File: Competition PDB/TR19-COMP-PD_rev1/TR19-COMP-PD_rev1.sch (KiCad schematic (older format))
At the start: 38 parts

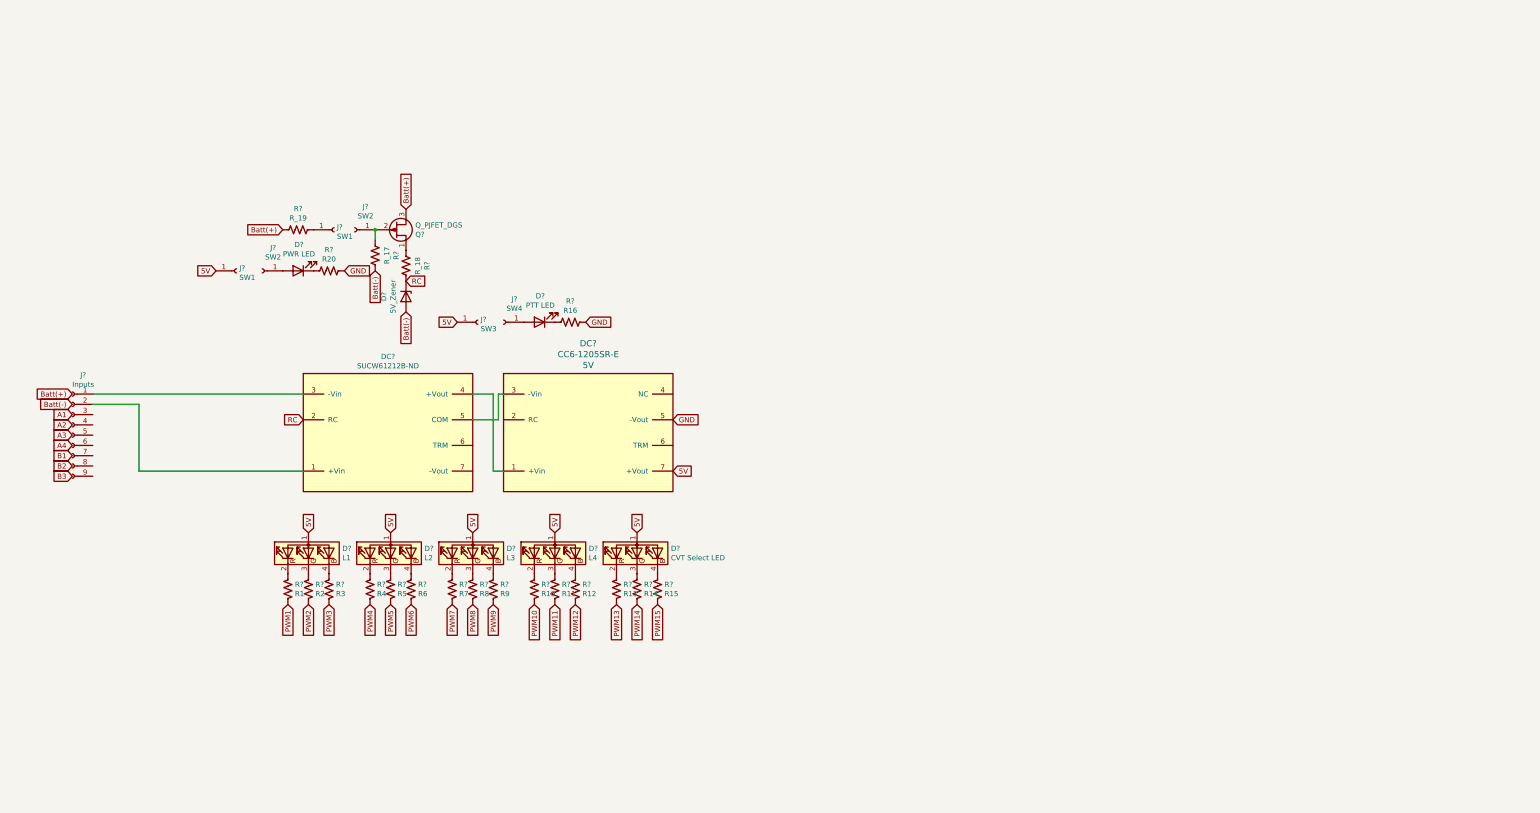
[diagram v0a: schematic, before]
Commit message: Baja Competition PCBs
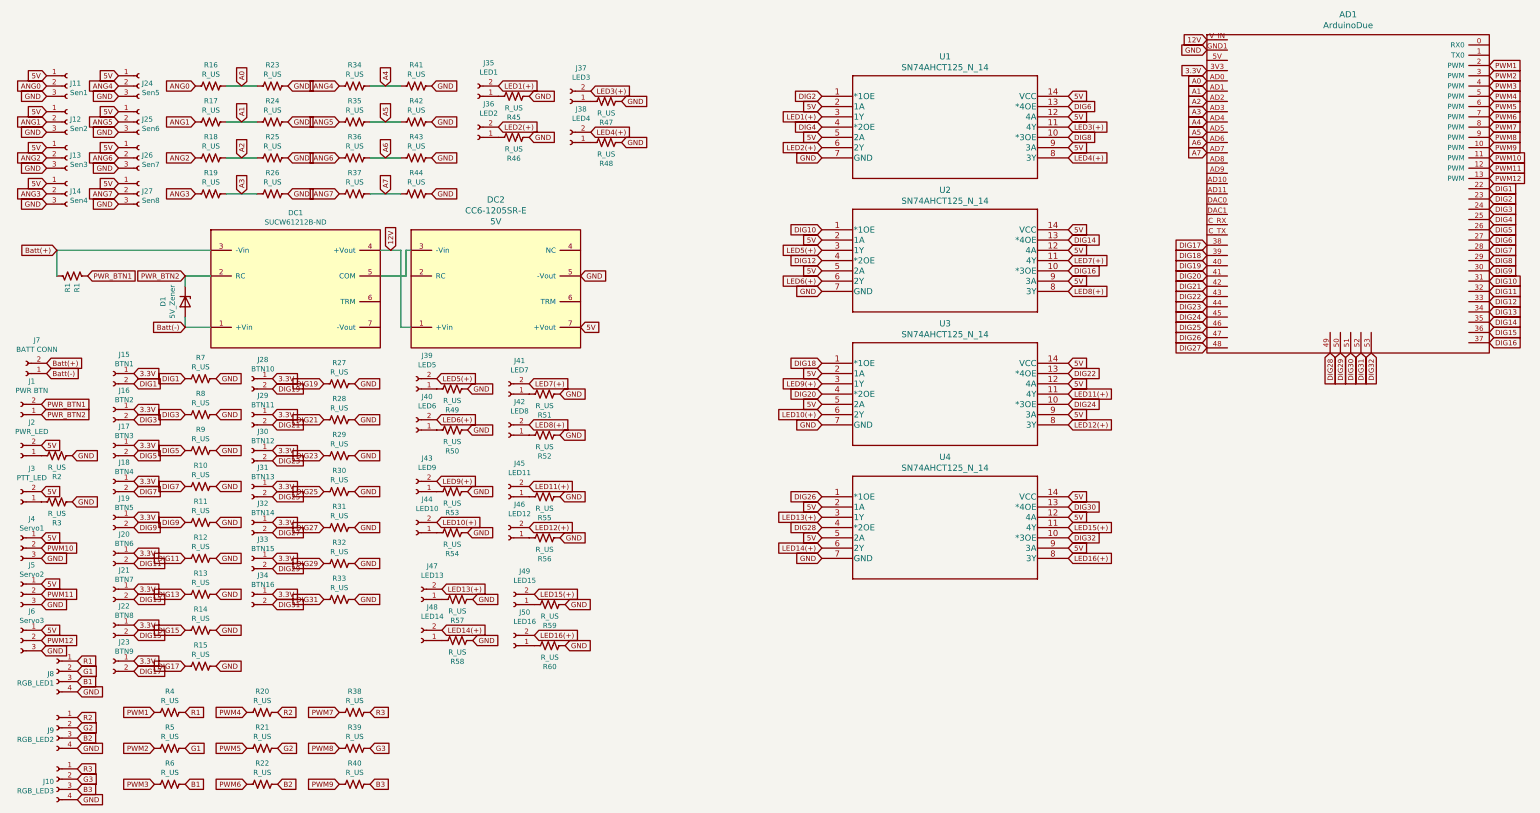
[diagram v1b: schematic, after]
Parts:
- removed D?: 5V_Zener, symbol Device:D_Zener
- removed D?: L1, symbol Device:LED_ARGB
- removed D?: L2, symbol Device:LED_ARGB
- removed D?: L3, symbol Device:LED_ARGB
- removed D?: L4, symbol Device:LED_ARGB
- removed D?: CVT Select LED, symbol Device:LED_ARGB
- removed D?: PTT LED, symbol Device:LED
- removed D?: PWR LED, symbol Device:LED
- removed J? (x2): SW1, symbol Connector:Conn_01x01_Female
- removed J? (x2): SW2, symbol Connector:Conn_01x01_Female
- removed J?: Inputs, symbol Connector:Conn_01x09_Female
- removed J?: SW3, symbol Connector:Conn_01x01_Female
- removed J?: SW4, symbol Connector:Conn_01x01_Female
- removed Q?: Q_PJFET_DGS, symbol Device:Q_PJFET_DGS
- removed R?: R_19, symbol Device:R_US
- removed R?: R1, symbol Device:R_US
- removed R?: R2, symbol Device:R_US
- removed R?: R3, symbol Device:R_US
- removed R?: R4, symbol Device:R_US
- removed R?: R5, symbol Device:R_US
- removed R?: R6, symbol Device:R_US
- removed R?: R7, symbol Device:R_US
- removed R?: R8, symbol Device:R_US
- removed R?: R9, symbol Device:R_US
- removed R?: R10, symbol Device:R_US
- removed R?: R11, symbol Device:R_US
- removed R?: R12, symbol Device:R_US
- removed R?: R13, symbol Device:R_US
- removed R?: R14, symbol Device:R_US
- removed R?: R15, symbol Device:R_US
- removed R?: R16, symbol Device:R_US
- removed R?: R_17, symbol Device:R_US
- removed R?: R_18, symbol Device:R_US
- removed R?: R20, symbol Device:R_US
- added AD1: ArduinoDue, TR_Library:ARDUINO_DUE_SHIELD_V2, symbol TR-Baja-Components:ArduinoDue
- added D1: 5V_Zener, Diode_SMD:D_0603_1608Metric_Pad1.05x0.95mm_HandSolder, symbol Device:D_Zener
- added J1: PWR BTN, Connector_PinHeader_2.54mm:PinHeader_1x02_P2.54mm_Vertical, symbol Connector:Conn_01x02_Female
- added J10: RGB_LED3, Connector_PinHeader_2.54mm:PinHeader_1x04_P2.54mm_Vertical, symbol Connector:Conn_01x04_Female
- added J11: Sen1, Connector_PinHeader_2.54mm:PinHeader_1x03_P2.54mm_Vertical, symbol Connector:Conn_01x03_Female
- added J12: Sen2, Connector_PinHeader_2.54mm:PinHeader_1x03_P2.54mm_Vertical, symbol Connector:Conn_01x03_Female
- added J13: Sen3, Connector_PinHeader_2.54mm:PinHeader_1x03_P2.54mm_Vertical, symbol Connector:Conn_01x03_Female
- added J14: Sen4, Connector_PinHeader_2.54mm:PinHeader_1x03_P2.54mm_Vertical, symbol Connector:Conn_01x03_Female
- added J15: BTN1, Connector_PinHeader_2.54mm:PinHeader_1x02_P2.54mm_Vertical, symbol Connector:Conn_01x02_Female
- added J16: BTN2, Connector_PinHeader_2.54mm:PinHeader_1x02_P2.54mm_Vertical, symbol Connector:Conn_01x02_Female
- added J17: BTN3, Connector_PinHeader_2.54mm:PinHeader_1x02_P2.54mm_Vertical, symbol Connector:Conn_01x02_Female
- added J18: BTN4, Connector_PinHeader_2.54mm:PinHeader_1x02_P2.54mm_Vertical, symbol Connector:Conn_01x02_Female
- added J19: BTN5, Connector_PinHeader_2.54mm:PinHeader_1x02_P2.54mm_Vertical, symbol Connector:Conn_01x02_Female
- added J2: PWR_LED, Connector_PinHeader_2.54mm:PinHeader_1x02_P2.54mm_Vertical, symbol Connector:Conn_01x02_Female
- added J20: BTN6, Connector_PinHeader_2.54mm:PinHeader_1x02_P2.54mm_Vertical, symbol Connector:Conn_01x02_Female
- added J21: BTN7, Connector_PinHeader_2.54mm:PinHeader_1x02_P2.54mm_Vertical, symbol Connector:Conn_01x02_Female
- added J22: BTN8, Connector_PinHeader_2.54mm:PinHeader_1x02_P2.54mm_Vertical, symbol Connector:Conn_01x02_Female
- added J23: BTN9, Connector_PinHeader_2.54mm:PinHeader_1x02_P2.54mm_Vertical, symbol Connector:Conn_01x02_Female
- added J24: Sen5, Connector_PinHeader_2.54mm:PinHeader_1x03_P2.54mm_Vertical, symbol Connector:Conn_01x03_Female
- added J25: Sen6, Connector_PinHeader_2.54mm:PinHeader_1x03_P2.54mm_Vertical, symbol Connector:Conn_01x03_Female
- added J26: Sen7, Connector_PinHeader_2.54mm:PinHeader_1x03_P2.54mm_Vertical, symbol Connector:Conn_01x03_Female
- added J27: Sen8, Connector_PinHeader_2.54mm:PinHeader_1x03_P2.54mm_Vertical, symbol Connector:Conn_01x03_Female
- added J28: BTN10, Connector_PinHeader_2.54mm:PinHeader_1x02_P2.54mm_Vertical, symbol Connector:Conn_01x02_Female
- added J29: BTN11, Connector_PinHeader_2.54mm:PinHeader_1x02_P2.54mm_Vertical, symbol Connector:Conn_01x02_Female
- added J3: PTT_LED, Connector_PinHeader_2.54mm:PinHeader_1x02_P2.54mm_Vertical, symbol Connector:Conn_01x02_Female
- added J30: BTN12, Connector_PinHeader_2.54mm:PinHeader_1x02_P2.54mm_Vertical, symbol Connector:Conn_01x02_Female
- added J31: BTN13, Connector_PinHeader_2.54mm:PinHeader_1x02_P2.54mm_Vertical, symbol Connector:Conn_01x02_Female
- added J32: BTN14, Connector_PinHeader_2.54mm:PinHeader_1x02_P2.54mm_Vertical, symbol Connector:Conn_01x02_Female
- added J33: BTN15, Connector_PinHeader_2.54mm:PinHeader_1x02_P2.54mm_Vertical, symbol Connector:Conn_01x02_Female
- added J34: BTN16, Connector_PinHeader_2.54mm:PinHeader_1x02_P2.54mm_Vertical, symbol Connector:Conn_01x02_Female
- added J35: LED1, Connector_PinHeader_2.54mm:PinHeader_1x02_P2.54mm_Vertical, symbol Connector:Conn_01x02_Female
- added J36: LED2, Connector_PinHeader_2.54mm:PinHeader_1x02_P2.54mm_Vertical, symbol Connector:Conn_01x02_Female
- added J37: LED3, Connector_PinHeader_2.54mm:PinHeader_1x02_P2.54mm_Vertical, symbol Connector:Conn_01x02_Female
- added J38: LED4, Connector_PinHeader_2.54mm:PinHeader_1x02_P2.54mm_Vertical, symbol Connector:Conn_01x02_Female
- added J39: LED5, Connector_PinHeader_2.54mm:PinHeader_1x02_P2.54mm_Vertical, symbol Connector:Conn_01x02_Female
- added J4: Servo1, Connector_PinHeader_2.54mm:PinHeader_1x03_P2.54mm_Vertical, symbol Connector:Conn_01x03_Female
- added J40: LED6, Connector_PinHeader_2.54mm:PinHeader_1x02_P2.54mm_Vertical, symbol Connector:Conn_01x02_Female
- added J41: LED7, Connector_PinHeader_2.54mm:PinHeader_1x02_P2.54mm_Vertical, symbol Connector:Conn_01x02_Female
- added J42: LED8, Connector_PinHeader_2.54mm:PinHeader_1x02_P2.54mm_Vertical, symbol Connector:Conn_01x02_Female
- added J43: LED9, Connector_PinHeader_2.54mm:PinHeader_1x02_P2.54mm_Vertical, symbol Connector:Conn_01x02_Female
- added J44: LED10, Connector_PinHeader_2.54mm:PinHeader_1x02_P2.54mm_Vertical, symbol Connector:Conn_01x02_Female
- added J45: LED11, Connector_PinHeader_2.54mm:PinHeader_1x02_P2.54mm_Vertical, symbol Connector:Conn_01x02_Female
- added J46: LED12, Connector_PinHeader_2.54mm:PinHeader_1x02_P2.54mm_Vertical, symbol Connector:Conn_01x02_Female
- added J47: LED13, Connector_PinHeader_2.54mm:PinHeader_1x02_P2.54mm_Vertical, symbol Connector:Conn_01x02_Female
- added J48: LED14, Connector_PinHeader_2.54mm:PinHeader_1x02_P2.54mm_Vertical, symbol Connector:Conn_01x02_Female
- added J49: LED15, Connector_PinHeader_2.54mm:PinHeader_1x02_P2.54mm_Vertical, symbol Connector:Conn_01x02_Female
- added J5: Servo2, Connector_PinHeader_2.54mm:PinHeader_1x03_P2.54mm_Vertical, symbol Connector:Conn_01x03_Female
- added J50: LED16, Connector_PinHeader_2.54mm:PinHeader_1x02_P2.54mm_Vertical, symbol Connector:Conn_01x02_Female
- added J6: Servo3, Connector_PinHeader_2.54mm:PinHeader_1x03_P2.54mm_Vertical, symbol Connector:Conn_01x03_Female
- added J7: BATT CONN, Connector_PinHeader_2.54mm:PinHeader_1x02_P2.54mm_Vertical, symbol Connector:Conn_01x02_Female
- added J8: RGB_LED1, Connector_PinHeader_2.54mm:PinHeader_1x04_P2.54mm_Vertical, symbol Connector:Conn_01x04_Female
- added J9: RGB_LED2, Connector_PinHeader_2.54mm:PinHeader_1x04_P2.54mm_Vertical, symbol Connector:Conn_01x04_Female
- added R1: R1, Resistor_SMD:R_1210_3225Metric_Pad1.42x2.65mm_HandSolder, symbol Device:R_US
- added R10, R11, R12, R13, R14, R15, R16, R17, R18, R19, R2, R20, R21, R22, R23, R24, R25, R26, R27, R28, R29, R3, R30, R31, R32, R33, R34, R35, R36, R37, R38, R39, R4, R40, R41, R42, R43, R44, R45, R46, R47, R48, R49, R5, R50, R51, R52, R53, R54, R55, R56, R57, R58, R59, R6, R60, R7, R8, R9: R_US, Resistor_SMD:R_1210_3225Metric_Pad1.42x2.65mm_HandSolder, symbol Device:R_US
- added U1, U2, U3, U4: SN74AHCT125_N_14, TR_Library:SN74AHCT125N, symbol TR-Baja-Components:SN74AHCT125_N_14
- DC1: renamed from DC?; footprint (none) -> TR_Library:1776-2753-ND
- DC2: renamed from DC?; footprint (none) -> TR_Library:445-2487-ND
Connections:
- net 5V: now also J11.1 (Pin_1), J12.1 (Pin_1), J13.1 (Pin_1), J14.1 (Pin_1), J2.2 (Pin_2), J24.1 (Pin_1), J25.1 (Pin_1), J26.1 (Pin_1), J27.1 (Pin_1), J3.2 (Pin_2), J4.1 (Pin_1), J5.1 (Pin_1), J6.1 (Pin_1), U1.12 (4A), U1.14 (VCC), U1.2 (1A), U1.5 (2A), U1.9 (3A), U2.12 (4A), U2.14 (VCC), U2.2 (1A), U2.5 (2A), U2.9 (3A), U3.12 (4A), U3.14 (VCC), U3.2 (1A), U3.5 (2A), U3.9 (3A), U4.12 (4A), U4.14 (VCC), U4.2 (1A), U4.5 (2A), U4.9 (3A)
- net A1: now also AD1.AD1, R17.1, R24.2
- net A2: now also AD1.AD2, R18.1, R25.2
- net A3: now also AD1.AD3, R19.1, R26.2
- net A4: now also AD1.AD4, R34.1, R41.2
- net B1: now also J8.3 (Pin_3), R6.1
- net B2: now also J9.3 (Pin_3), R22.1
- net B3: now also J10.3 (Pin_3), R40.1
- net Batt(+): now also DC1.3 (-Vin), J7.2 (Pin_2), R1.2
- net Batt(-): now also DC1.1 (+Vin), D1.2 (A), J7.1 (Pin_1)
- net GND: now also AD1.GND1, J10.4 (Pin_4), J11.3 (Pin_3), J12.3 (Pin_3), J13.3 (Pin_3), J14.3 (Pin_3), J24.3 (Pin_3), J25.3 (Pin_3), J26.3 (Pin_3), J27.3 (Pin_3), J4.3 (Pin_3), J5.3 (Pin_3), J6.3 (Pin_3), J8.4 (Pin_4), J9.4 (Pin_4), R10.1, R11.1, R12.1, R13.1, R14.1, R15.1, R2.2, R23.1, R24.1, R25.1, R26.1, R27.1, R28.1, R29.1, R3.2, R30.1, R31.1, R32.1, R33.1, R41.1, R42.1, R43.1, R44.1, R45.2, R46.2, R47.2, R48.2, R49.2, R50.2, R51.2, R52.2, R53.2, R54.2, R55.2, R56.2, R57.2, R58.2, R59.2, R60.2, R7.1, R8.1, R9.1, U1.7 (GND), U2.7 (GND), U3.7 (GND), U4.7 (GND)
- net PWM1: now also AD1.2 (PWM), R4.2
- net PWM10: now also AD1.11 (PWM), J4.2 (Pin_2)
- net PWM11: now also AD1.12 (PWM), J5.2 (Pin_2)
- net PWM12: now also AD1.13 (PWM), J6.2 (Pin_2)
- net PWM2: now also AD1.3 (PWM), R5.2
- net PWM3: now also AD1.4 (PWM), R6.2
- net PWM4: now also AD1.5 (PWM), R20.2
- net PWM5: now also AD1.6 (PWM), R21.2
- net PWM6: now also AD1.7 (PWM), R22.2
- net PWM7: now also AD1.8 (PWM), R38.2
- net PWM8: now also AD1.9 (PWM), R39.2
- net PWM9: now also AD1.10 (PWM), R40.2
- net 12V: now reaches DC1.4 (+Vout), DC2.1 (+Vin)
- net 12V: now also AD1.V_IN
- net RC renamed PWR_BTN2
- net PWR_BTN2: now also D1.1 (K), J1.1 (Pin_1)
- new net: J2.1 (Pin_1), R2.1
- new net: J3.1 (Pin_1), R3.1
- new net: J35.1 (Pin_1), R45.1
- new net: J36.1 (Pin_1), R46.1
- new net: J37.1 (Pin_1), R47.1
- new net: J38.1 (Pin_1), R48.1
- new net: J39.1 (Pin_1), R49.1
- new net: J40.1 (Pin_1), R50.1
- new net: J41.1 (Pin_1), R51.1
- new net: J42.1 (Pin_1), R52.1
- new net: J43.1 (Pin_1), R53.1
- new net: J44.1 (Pin_1), R54.1
- new net: J45.1 (Pin_1), R55.1
- new net: J46.1 (Pin_1), R56.1
- new net: J47.1 (Pin_1), R57.1
- new net: J48.1 (Pin_1), R58.1
- new net: J49.1 (Pin_1), R59.1
- new net: J50.1 (Pin_1), R60.1
- new net 3.3V: AD1.3V3, J15.1 (Pin_1), J16.1 (Pin_1), J17.1 (Pin_1), J18.1 (Pin_1), J19.1 (Pin_1), J20.1 (Pin_1), J21.1 (Pin_1), J22.1 (Pin_1), J23.1 (Pin_1), J28.1 (Pin_1), J29.1 (Pin_1), J30.1 (Pin_1), J31.1 (Pin_1), J32.1 (Pin_1), J33.1 (Pin_1), J34.1 (Pin_1)
- new net A0: AD1.AD0, R16.1, R23.2
- new net A5: AD1.AD5, R35.1, R42.2
- new net A6: AD1.AD6, R36.1, R43.2
- new net A7: AD1.AD7, R37.1, R44.2
- new net ANG0: J11.2 (Pin_2), R16.2
- new net ANG1: J12.2 (Pin_2), R17.2
- new net ANG2: J13.2 (Pin_2), R18.2
- new net ANG3: J14.2 (Pin_2), R19.2
- new net ANG4: J24.2 (Pin_2), R34.2
- new net ANG5: J25.2 (Pin_2), R35.2
- new net ANG6: J26.2 (Pin_2), R36.2
- new net ANG7: J27.2 (Pin_2), R37.2
- new net DIG1: AD1.22, J15.2 (Pin_2), R7.2
- new net DIG10: AD1.31, U2.1 (*1OE)
- new net DIG11: AD1.32, J20.2 (Pin_2), R12.2
- new net DIG12: AD1.33, U2.4 (*2OE)
- new net DIG13: AD1.34, J21.2 (Pin_2), R13.2
- new net DIG14: AD1.35, U2.13 (*4OE)
- new net DIG15: AD1.36, J22.2 (Pin_2), R14.2
- new net DIG16: AD1.37, U2.10 (*3OE)
- new net DIG17: AD1.38, J23.2 (Pin_2), R15.2
- new net DIG18: AD1.39, U3.1 (*1OE)
- new net DIG19: AD1.40, J28.2 (Pin_2), R27.2
- new net DIG2: AD1.23, U1.1 (*1OE)
- new net DIG20: AD1.41, U3.4 (*2OE)
- new net DIG21: AD1.42, J29.2 (Pin_2), R28.2
- new net DIG22: AD1.43, U3.13 (*4OE)
- new net DIG23: AD1.44, J30.2 (Pin_2), R29.2
- new net DIG24: AD1.45, U3.10 (*3OE)
- new net DIG25: AD1.46, J31.2 (Pin_2), R30.2
- new net DIG26: AD1.47, U4.1 (*1OE)
- new net DIG27: AD1.48, J32.2 (Pin_2), R31.2
- new net DIG28: AD1.49, U4.4 (*2OE)
- new net DIG29: AD1.50, J33.2 (Pin_2), R32.2
- new net DIG3: AD1.24, J16.2 (Pin_2), R8.2
- new net DIG30: AD1.51, U4.13 (*4OE)
- new net DIG31: AD1.52, J34.2 (Pin_2), R33.2
- new net DIG32: AD1.53, U4.10 (*3OE)
- new net DIG4: AD1.25, U1.4 (*2OE)
- new net DIG5: AD1.26, J17.2 (Pin_2), R9.2
- new net DIG6: AD1.27, U1.13 (*4OE)
- new net DIG7: AD1.28, J18.2 (Pin_2), R10.2
- new net DIG8: AD1.29, U1.10 (*3OE)
- new net DIG9: AD1.30, J19.2 (Pin_2), R11.2
- new net G1: J8.2 (Pin_2), R5.1
- new net G2: J9.2 (Pin_2), R21.1
- new net G3: J10.2 (Pin_2), R39.1
- new net LED1(+): J35.2 (Pin_2), U1.3 (1Y)
- new net LED10(+): J44.2 (Pin_2), U3.6 (2Y)
- new net LED11(+): J45.2 (Pin_2), U3.11 (4Y)
- new net LED12(+): J46.2 (Pin_2), U3.8 (3Y)
- new net LED13(+): J47.2 (Pin_2), U4.3 (1Y)
- new net LED14(+): J48.2 (Pin_2), U4.6 (2Y)
- new net LED15(+): J49.2 (Pin_2), U4.11 (4Y)
- new net LED16(+): J50.2 (Pin_2), U4.8 (3Y)
- new net LED2(+): J36.2 (Pin_2), U1.6 (2Y)
- new net LED3(+): J37.2 (Pin_2), U1.11 (4Y)
- new net LED4(+): J38.2 (Pin_2), U1.8 (3Y)
- new net LED5(+): J39.2 (Pin_2), U2.3 (1Y)
- new net LED6(+): J40.2 (Pin_2), U2.6 (2Y)
- new net LED7(+): J41.2 (Pin_2), U2.11 (4Y)
- new net LED8(+): J42.2 (Pin_2), U2.8 (3Y)
- new net LED9(+): J43.2 (Pin_2), U3.3 (1Y)
- new net PWR_BTN1: J1.2 (Pin_2), R1.1
- new net R1: J8.1 (Pin_1), R4.1
- new net R2: J9.1 (Pin_1), R20.1
- new net R3: J10.1 (Pin_1), R38.1
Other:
- moved on the sheet: DC1, DC2

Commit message: V2
Version 2 Final update
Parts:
- AD1: symbol TR-Baja-Components:ArduinoDue -> TR19-COMP-PD_rev1-rescue:ArduinoDue-TR-Baja-Components
- DC1: symbol TR-Baja-Components:SUCW61212B-ND -> TR19-COMP-PD_rev1-rescue:SUCW61212B-ND-TR-Baja-Components
- DC2: symbol TR-Baja-Components:CC6-1205SR-E -> TR19-COMP-PD_rev1-rescue:CC6-1205SR-E-TR-Baja-Components
- U1, U2, U3, U4: symbol TR-Baja-Components:SN74AHCT125_N_14 -> TR19-COMP-PD_rev1-rescue:SN74AHCT125_N_14-TR-Baja-Components
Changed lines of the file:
@@
 EESchema Schematic File Version 4
 LIBS:TR19-COMP-PD_rev1-cache
-EELAYER 26 0
+EELAYER 29 0
 EELAYER END
 $Descr A4 11693 8268
@@
 $EndDescr
 $Comp
-L TR-Baja-Components:SUCW61212B-ND DC1
+L TR19-COMP-PD_rev1-rescue:SUCW61212B-ND-TR-Baja-Components DC1
 U 1 1 5C786F0C
 P 3250 2700
@@
 $EndComp
 $Comp
-L TR-Baja-Components:CC6-1205SR-E DC2
+L TR19-COMP-PD_rev1-rescue:CC6-1205SR-E-TR-Baja-Components DC2
 U 1 1 5C786FA9
 P 5200 2700
@@
 PWR_BTN2
 $Comp
-L TR-Baja-Components:ArduinoDue AD1
+L TR19-COMP-PD_rev1-rescue:ArduinoDue-TR-Baja-Components AD1
 U 1 1 5CB9316F
 P 14050 2300
@@
 3.3V
 $Comp
-L TR-Baja-Components:SN74AHCT125_N_14 U1
+L TR19-COMP-PD_rev1-rescue:SN74AHCT125_N_14-TR-Baja-Components U1
 U 1 1 5CBD3AB0
 P 8350 850
@@
 GND
 $Comp
-L TR-Baja-Components:SN74AHCT125_N_14 U2
+L TR19-COMP-PD_rev1-rescue:SN74AHCT125_N_14-TR-Baja-Components U2
 U 1 1 5CBE249D
 P 8350 2150
@@
 GND
 $Comp
-L TR-Baja-Components:SN74AHCT125_N_14 U3
+L TR19-COMP-PD_rev1-rescue:SN74AHCT125_N_14-TR-Baja-Components U3
 U 1 1 5CBE7459
 P 8350 3450
@@
 GND
 $Comp
-L TR-Baja-Components:SN74AHCT125_N_14 U4
+L TR19-COMP-PD_rev1-rescue:SN74AHCT125_N_14-TR-Baja-Components U4
 U 1 1 5CBEA6A8
 P 8350 4750
